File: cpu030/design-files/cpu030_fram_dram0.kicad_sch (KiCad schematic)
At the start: 45 parts, among them J201 DRAM0SZ, J202 DRAM0 JTAG, U201 ATF1508AS, U202 CY7C1061GE (U16), U203 CY7C1061GE (L16), U204 SIMM72-0A, U205 SIMM72-0B, U206 74ACT05

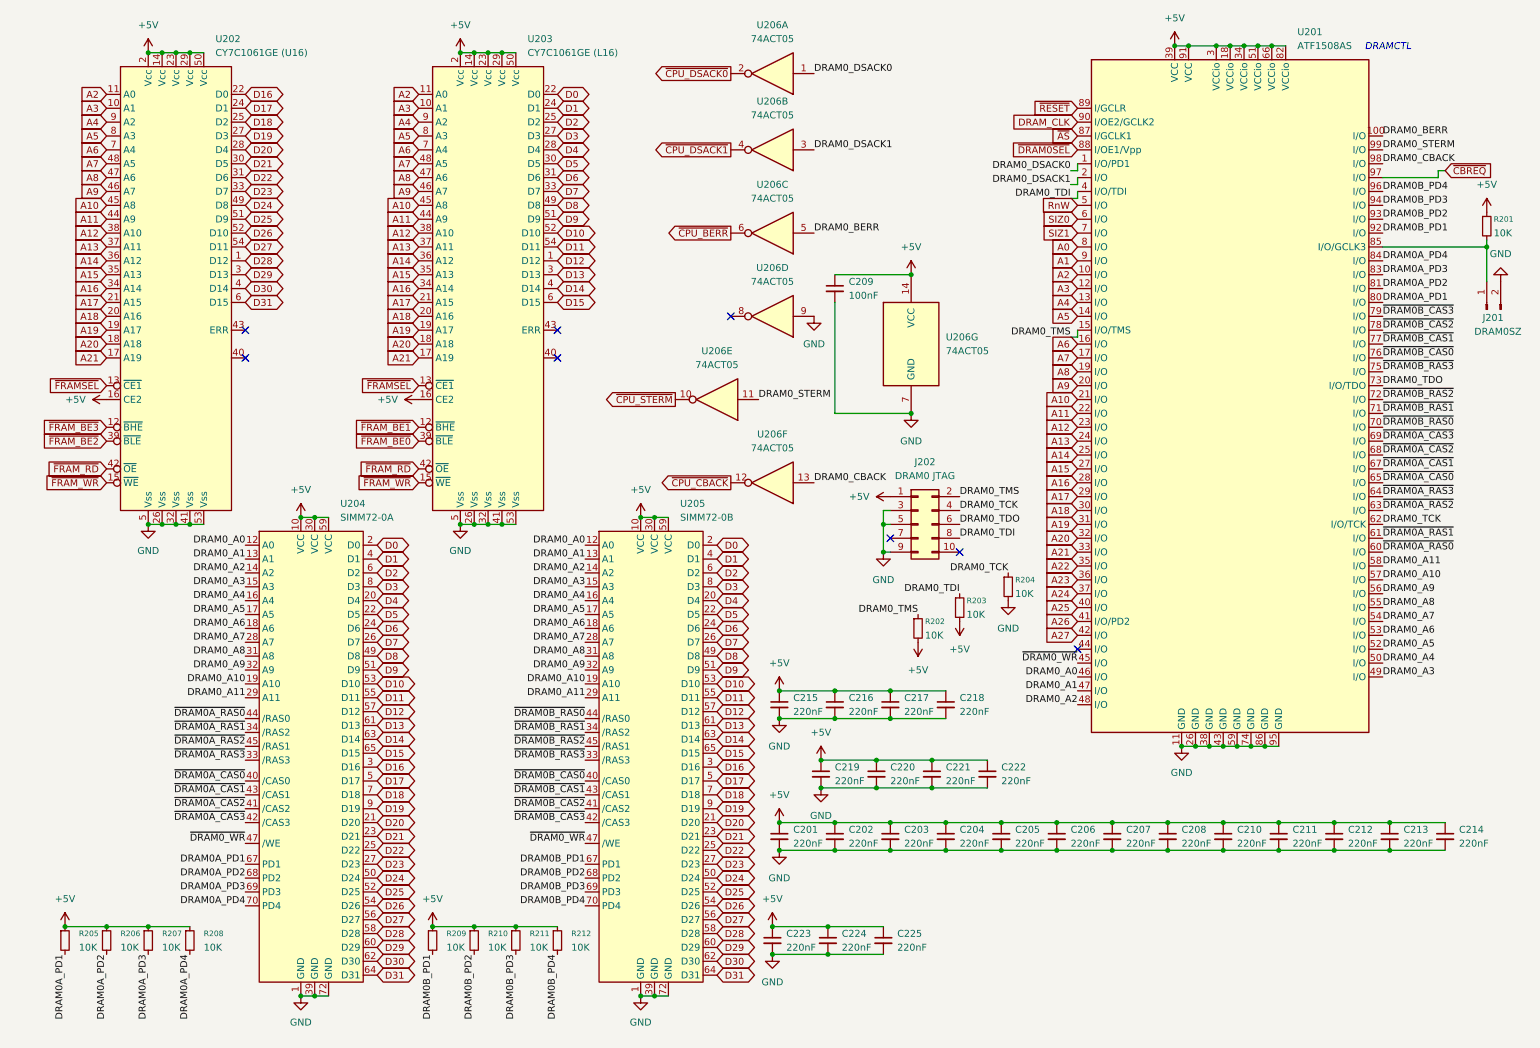
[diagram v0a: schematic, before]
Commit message: Fix silliness in the SIMM-72 symbol that tripped the ERC.
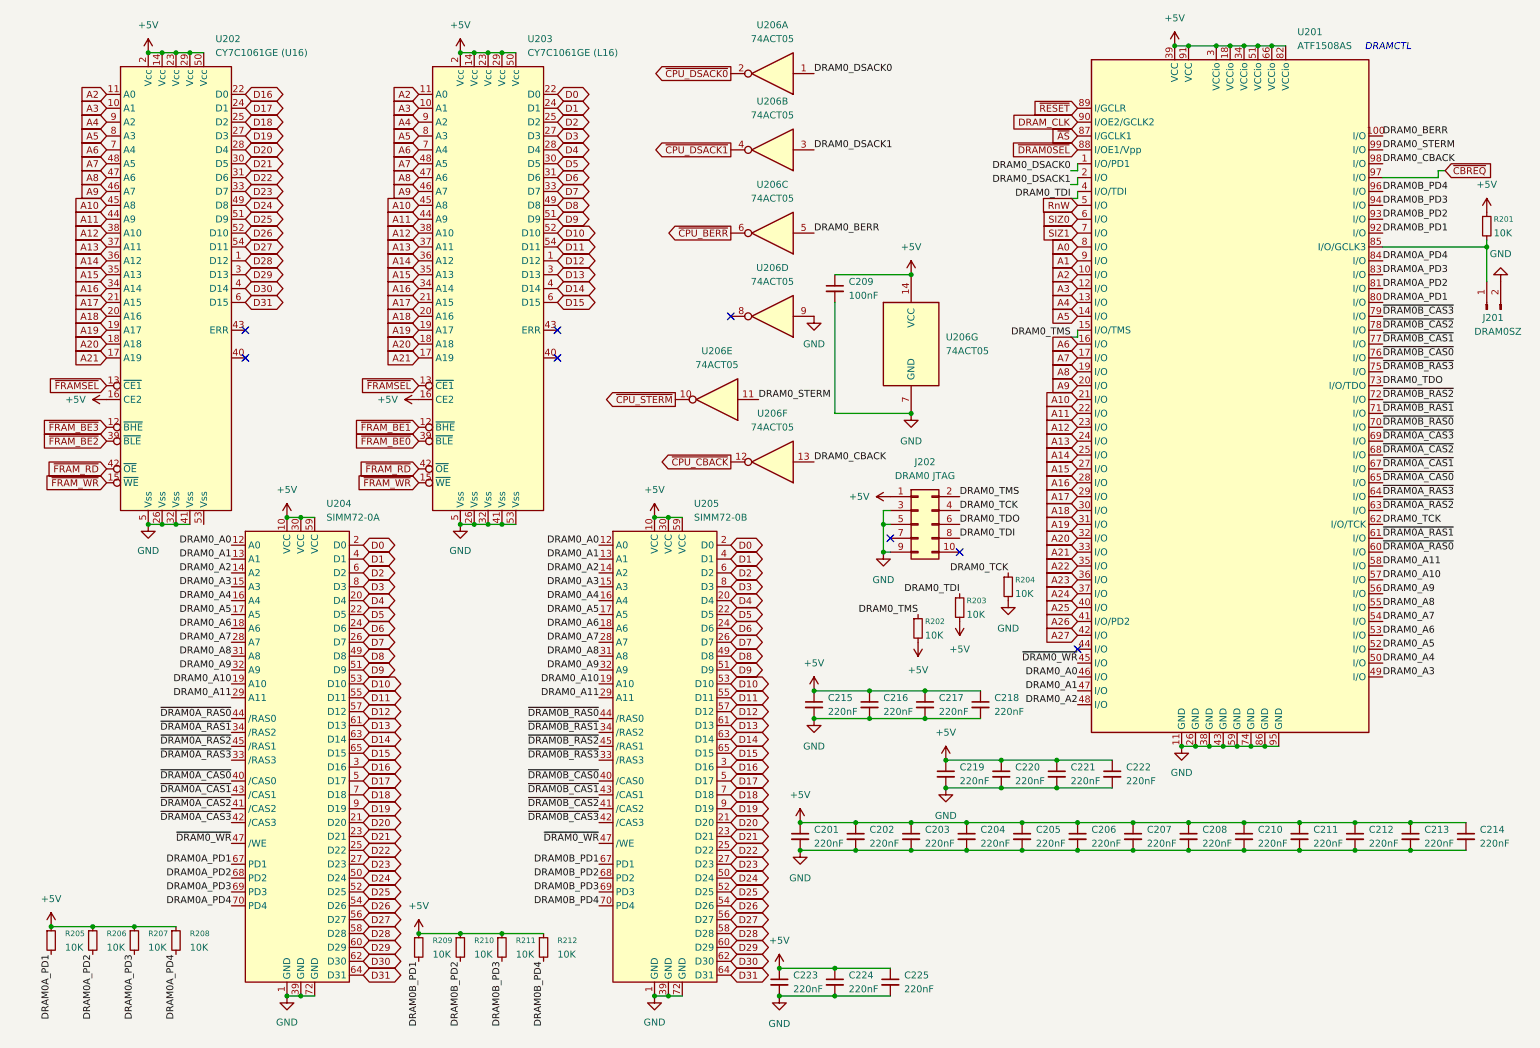
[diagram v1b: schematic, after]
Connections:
- net +5V: no longer U205.11 (NC)
- net DRAM0B_PD4: no longer U205.36 (NC)
- net GND: no longer U202.53 (Vss)
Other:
- moved on the sheet: C201, C202, C203, C204, C205, C206, C207, C208, C210, C211, C212, C213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
